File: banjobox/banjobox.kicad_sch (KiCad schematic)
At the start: 8 parts, among them SW1 RotaryEncoder_Switch, U1 SHT31-DIS, U2 MOUDLE-SEEEDUINO-XIAO, U3 ER_OLEDM0.91_1x-I2C, U4 PAM8302AAY

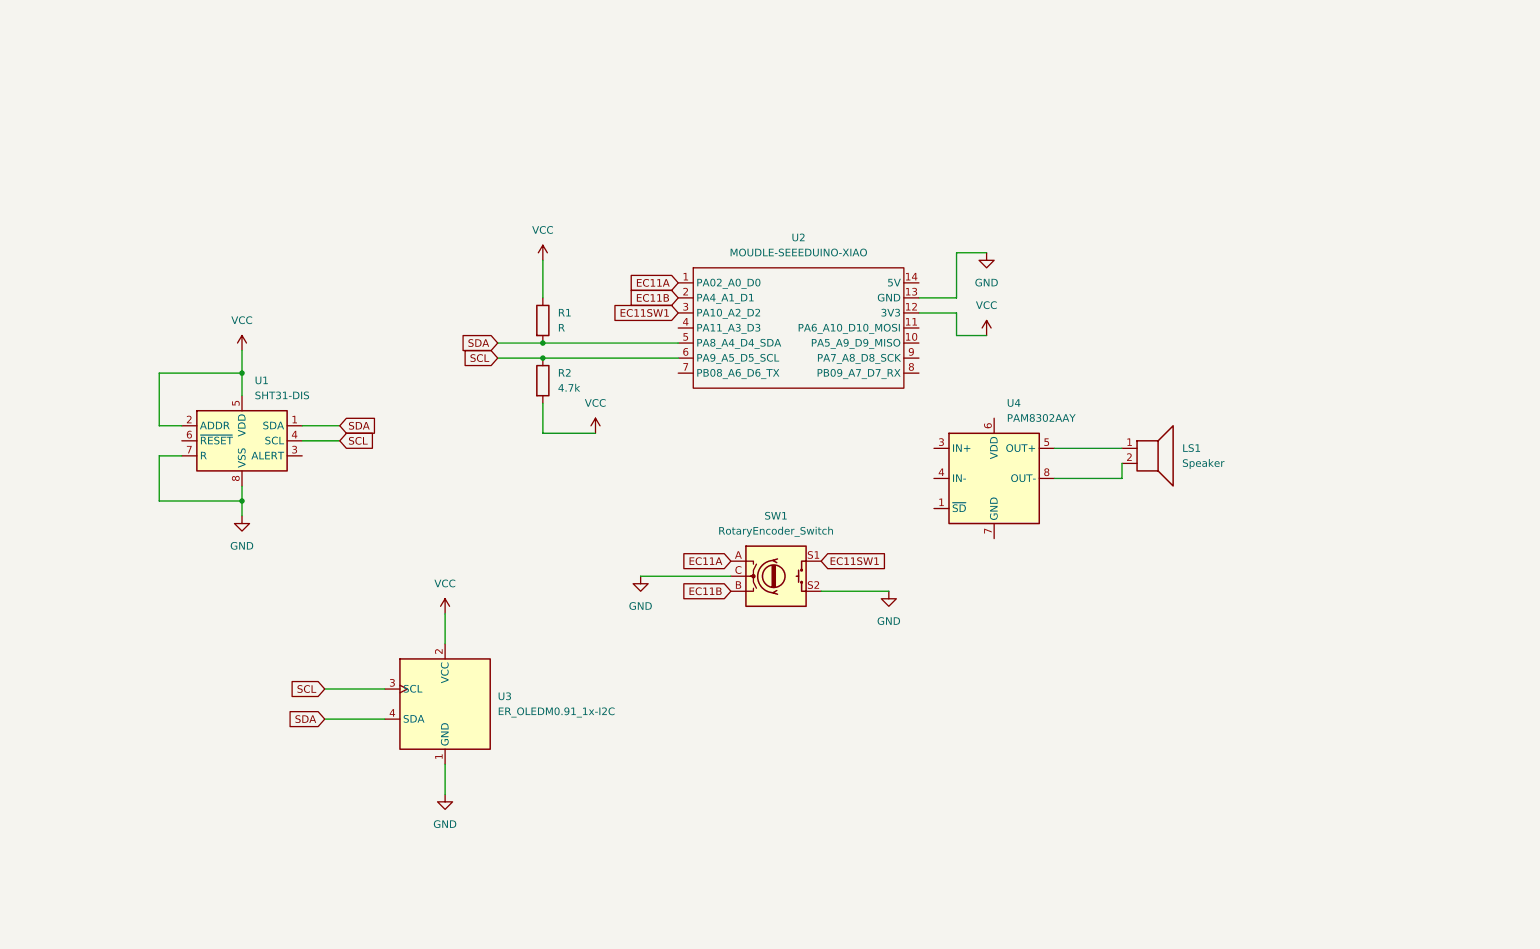
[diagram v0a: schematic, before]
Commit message: first draft of schematic
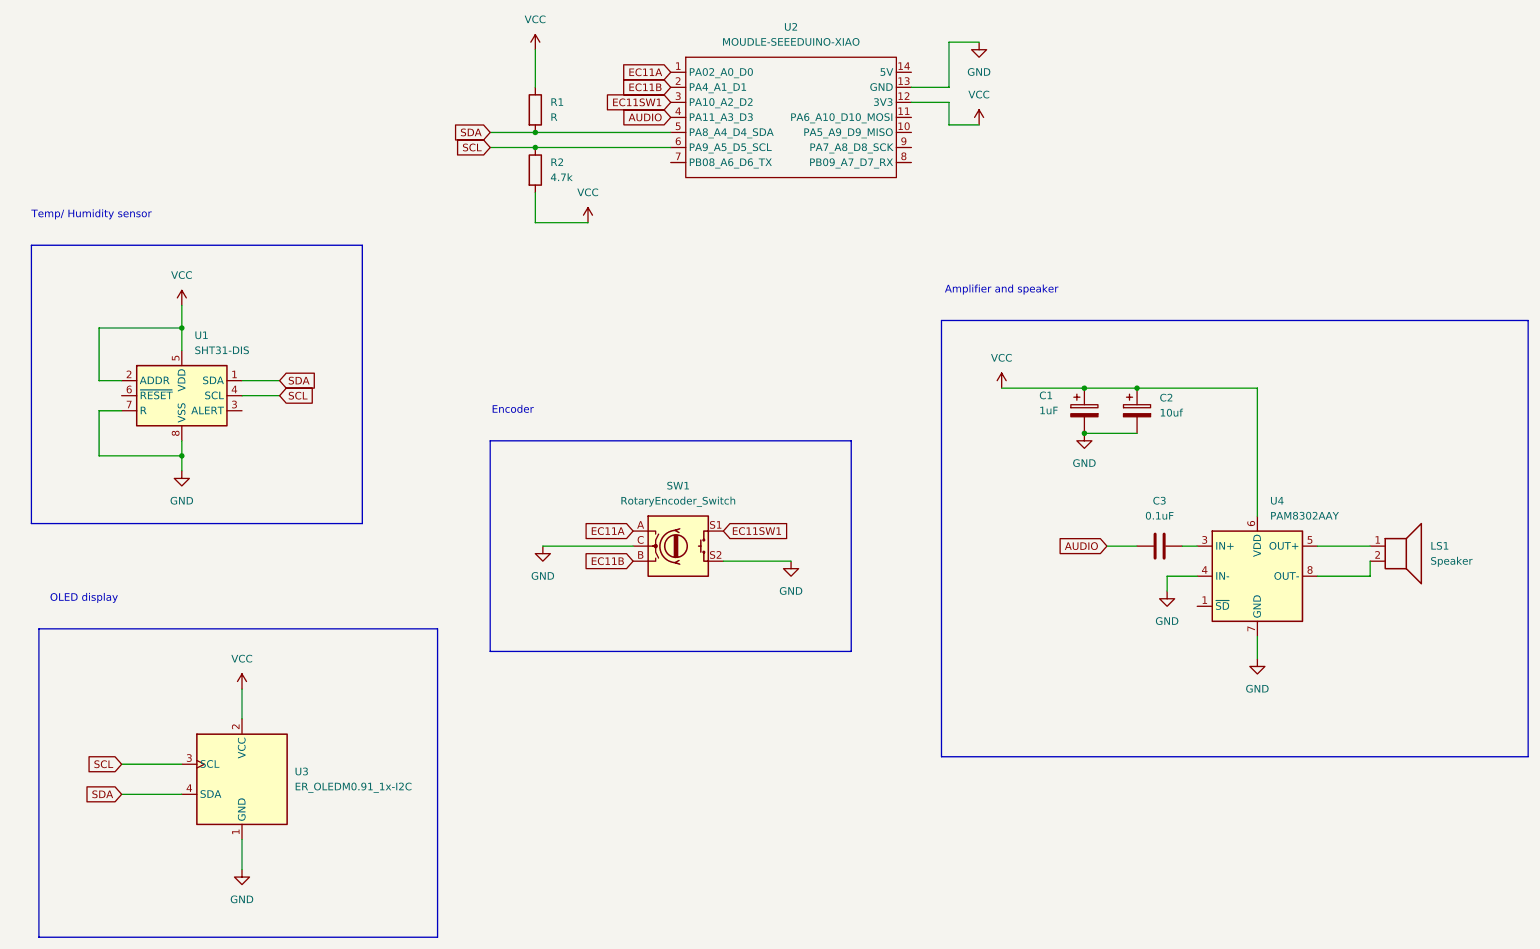
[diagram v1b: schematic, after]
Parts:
- added C1: 1uF, symbol Device:C_Polarized
- added C2: 10uf, symbol Device:C_Polarized
- added C3: 0.1uF, symbol Device:C
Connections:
- net GND: now also U4.4 (IN-), U4.7 (GND), C1.2, C2.2
- net VCC: now also U4.6 (VDD), C1.1, C2.1
- net at U4.3 (IN+): now also C3.2
- net AUDIO: now reaches U2.4 (PA11_A3_D3)
- net AUDIO: now also C3.1
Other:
- note added: "Amplifier and speaker"
- note added: "Encoder"
- note added: "OLED display"
- note added: "Temp/ Humidity sensor"
- moved on the sheet: LS1, R1, R2, SW1, U1, U2, U3, U4
